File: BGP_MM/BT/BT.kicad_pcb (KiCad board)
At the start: 2 copper layers, 26 x 26 mm, 36 parts, among them J1 Conn_01x02_Male, J2 Conn_01x02_Male, J3 Conn_01x04_Male, J4 Conn_01x04_Male, Q1 MMBF5457, U1 MC33178

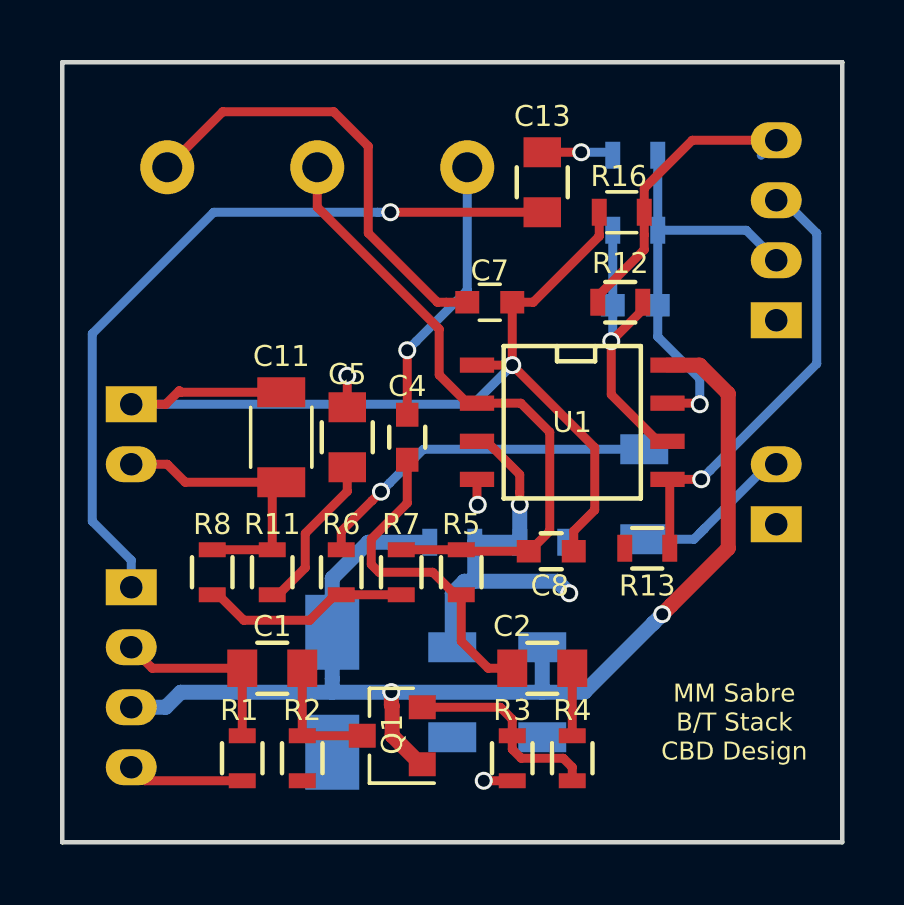
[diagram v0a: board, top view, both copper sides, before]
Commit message: MM Refactoring
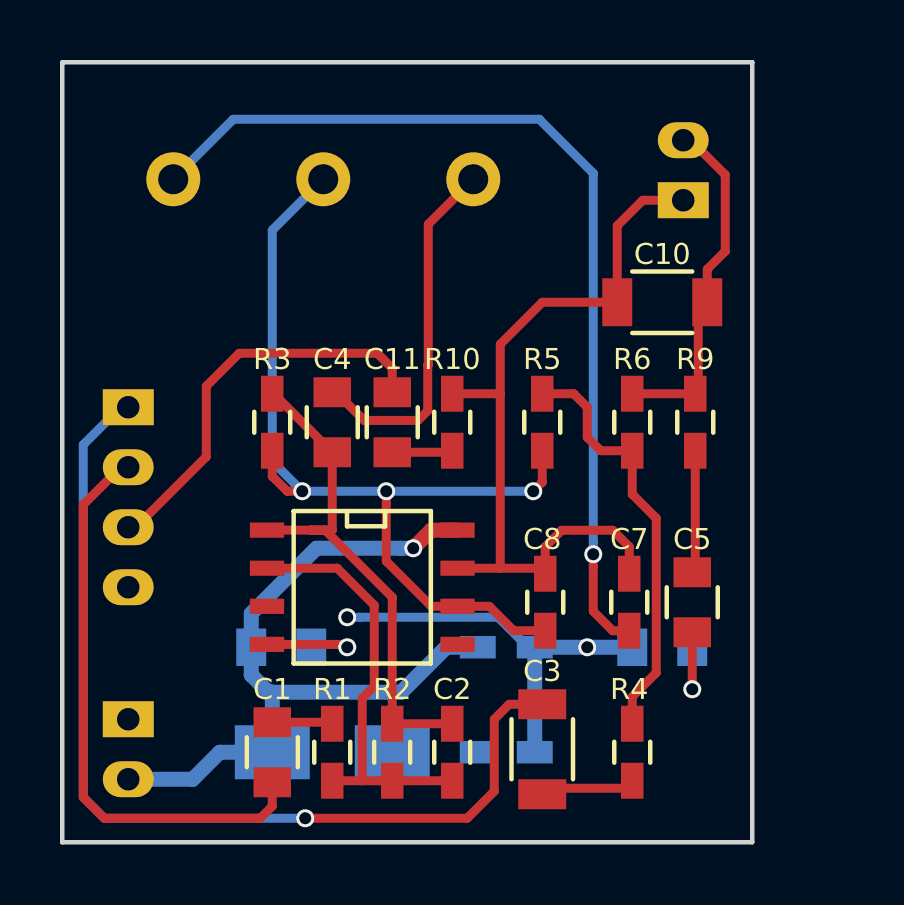
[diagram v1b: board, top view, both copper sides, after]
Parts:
- removed C12: 120p, Capacitors_SMD:C_0603
- removed C13: 1u, Capacitors_SMD:C_0805
- removed J4: Conn_01x04_Male, Connectors_JST:JST_PH_B4B-PH-K_04x2.00mm_Straight
- removed Q1: MMBF5457, TO_SOT_Packages_SMD:SOT-23
- removed R11: 10k, Resistors_SMD:R_0603
- removed R12, R14: 20k, Resistors_SMD:R_0603
- removed R13: 200k, Resistors_SMD:R_0603
- removed R15: 1k, Resistors_SMD:R_0603
- removed R16: 100, Resistors_SMD:R_0603
- added C10: 47n, Capacitors_SMD:C_1206, F.Cu at (165.0, 94.0)
- C1: value 0.1u -> 1u
- C11: value 47n -> 10u; footprint Capacitors_SMD:C_1206 -> Capacitors_SMD:C_0805
- C2: value 1u -> 120p; footprint Capacitors_SMD:C_0805 -> Capacitors_SMD:C_0603_HandSoldering
- C3: moved to F.Cu
- C4: footprint Capacitors_SMD:C_0603 -> Capacitors_SMD:C_0805
- C6, C9: value 47u -> 10u; footprint Capacitors_SMD:C_1206 -> Capacitors_SMD:C_0805
- C7, C8: footprint Capacitors_SMD:C_0603 -> Capacitors_SMD:C_0603_HandSoldering
- J2: value Conn_01x02_Male -> Conn_01x04_Male; footprint Connectors_JST:JST_PH_B2B-PH-K_02x2.00mm_Straight -> Connectors_JST:JST_PH_B4B-PH-K_04x2.00mm_Straight
- J3: value Conn_01x04_Male -> Conn_01x02_Male; footprint Connectors_JST:JST_PH_B4B-PH-K_04x2.00mm_Straight -> Connectors_JST:JST_PH_B2B-PH-K_02x2.00mm_Straight
- R1: footprint Resistors_SMD:R_0603 -> Capacitors_SMD:C_0603_HandSoldering
- R10: value 20k -> 1k; footprint Resistors_SMD:R_0603 -> Capacitors_SMD:C_0603_HandSoldering; moved to F.Cu
- R2: value 1MEG -> 470k; footprint Resistors_SMD:R_0603 -> Capacitors_SMD:C_0603_HandSoldering
- R3: value 20k -> 220k; footprint Resistors_SMD:R_0603 -> Capacitors_SMD:C_0603_HandSoldering
- R4: value 100 -> 1k; footprint Resistors_SMD:R_0603 -> Capacitors_SMD:C_0603_HandSoldering
- R5: value 220k -> 100k; footprint Resistors_SMD:R_0603 -> Capacitors_SMD:C_0603_HandSoldering
- R6: value 1k -> 2k; footprint Resistors_SMD:R_0603 -> Capacitors_SMD:C_0603_HandSoldering
- R7: footprint Resistors_SMD:R_0603 -> Capacitors_SMD:C_0603_HandSoldering; moved to B.Cu
- R8: value 2k -> 100k; footprint Resistors_SMD:R_0603 -> Capacitors_SMD:C_0603_HandSoldering; moved to B.Cu
- R9: value 20k -> 10k; footprint Resistors_SMD:R_0603 -> Capacitors_SMD:C_0603_HandSoldering; moved to F.Cu
- moved R3 13.8 mm to (152.0, 98.0), turned to 90 degrees
- moved C5 12.7 mm to (166.0, 104.0), turned to 270 degrees
- moved R8 11.5 mm to (159.8, 109.0), turned to 180 degrees
- moved J1 11.2 mm to (165.7, 90.6)
- moved C7 11.0 mm to (163.9, 104.0), turned to 90 degrees
- moved R6 10.9 mm to (164.0, 98.0), turned to 270 degrees
- moved C3 9.15 mm to (161.0, 108.9), turned to 90 degrees
- moved R9 9.03 mm to (166.1, 98.0), turned to 270 degrees
- moved U1 8.90 mm to (155.0, 103.5)
- moved C6 8.83 mm to (152.3, 105.5), turned to 0 degrees
- moved C9 7.16 mm to (165.0, 105.5), turned to 0 degrees
- moved R5 5.68 mm to (161.0, 98.0)
- moved R10 5.00 mm to (158.0, 98.0), turned to 90 degrees
- moved J3 4.40 mm to (147.2, 107.9)
- moved R7 4.30 mm to (159.8, 105.5), turned to 0 degrees
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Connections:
- C3 pad 2: Net-(C3-Pad2) -> /BR_O
- C4 pad 1: Net-(C2-Pad2) -> Net-(C2-Pad1)
- C7 pad 2: Net-(C11-Pad2) -> Net-(C10-Pad2)
- C8 pad 2: Net-(C11-Pad2) -> Net-(C10-Pad2)
- J1 pad 1: Earth -> Net-(C10-Pad2)
- J1 pad 2: Net-(C3-Pad2) -> Net-(C10-Pad1)
- J2 pad 1: Net-(C11-Pad2) -> /BR_O
- J2 pad 2: Net-(C11-Pad1) -> /SIG_I
- J3 pad 1: Net-(C13-Pad2) -> Earth
- J3 pad 2: /SIG_I -> VCC
- R1 pad 1: /SIG_I -> Net-(C2-Pad2)
- R1 pad 2: Earth -> Net-(C1-Pad1)
- R10 pad 1: /Vref -> Net-(C11-Pad1)
- R10 pad 2: Earth -> Net-(C10-Pad2)
- R2 pad 1: Net-(C1-Pad1) -> Net-(C2-Pad1)
- R2 pad 2: /Vref -> Net-(C2-Pad2)
- R3 pad 1: Net-(Q1-Pad2) -> Net-(C8-Pad1)
- R3 pad 2: Earth -> Net-(C2-Pad1)
- R4 pad 1: Net-(C2-Pad1) -> Net-(R4-Pad1)
- R4 pad 2: Net-(Q1-Pad2) -> Net-(C3-Pad1)
- R5 pad 1: Net-(C8-Pad1) -> Net-(R4-Pad1)
- R5 pad 2: Net-(C2-Pad2) -> Net-(C8-Pad1)
- R6 pad 1: Net-(R6-Pad1) -> Net-(C10-Pad1)
- R6 pad 2: Net-(C3-Pad1) -> Net-(R4-Pad1)
- R7 pad 1: Net-(R6-Pad1) -> VCC
- R7 pad 2: Net-(C8-Pad1) -> /Vref
- R8 pad 1: Net-(C11-Pad1) -> /Vref
- R8 pad 2: Net-(R6-Pad1) -> Earth
- R9 pad 1: VCC -> Net-(C10-Pad1)
- R9 pad 2: /Vref -> Net-(C5-Pad1)
- U1 pad 1: Net-(C11-Pad2) -> Net-(C2-Pad1)
- U1 pad 2: Net-(C8-Pad1) -> Net-(C2-Pad2)
- U1 pad 5: /Mr -> /Vref
- U1 pad 6: Net-(C12-Pad2) -> Net-(C8-Pad1)
- U1 pad 7: /Mo -> Net-(C10-Pad2)
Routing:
- net /BR_O: track 0.00 -> 32.6 mm, vias 0 -> 1
- net Net-(C10-Pad2): track 0.00 -> 26.7 mm
- net Net-(C13-Pad2): track 25.7 -> 0.00 mm, vias 1 -> 0
- net Net-(C11-Pad2): track 34.5 -> 13.6 mm, vias 1 -> 0
- net Net-(C7-Pad1): track 15.1 -> 31.6 mm, vias 0 -> 1
- net VCC: track 41.6 -> 25.7 mm, vias 2 -> 1
- net Net-(C2-Pad1): track 2.25 -> 17.4 mm
- net /Mr: track 15.1 -> 0.00 mm, vias 1 -> 0
- net /Mo: track 14.3 -> 0.00 mm, vias 1 -> 0
- net Net-(R4-Pad1): track 0.00 -> 14.1 mm
- net /SIG_I: track 6.24 -> 19.3 mm
- net Net-(C10-Pad1): track 0.00 -> 11.7 mm
- net /Mi: track 10.5 -> 0.00 mm
- net Net-(C12-Pad2): track 9.75 -> 0.00 mm, vias 1 -> 0
- net Net-(C8-Pad1): track 21.6 -> 31.3 mm, vias 0 -> 3
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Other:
- board size 26 x 26 mm -> 23 x 26 mm
- board text removed: "MM Sabre B/T Stack CBD Design"
